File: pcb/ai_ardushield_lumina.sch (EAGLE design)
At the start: 90 parts, among them J1 1X02ST, J2 1X01, J3 1X06, J4 1X08, J5 1X08, J6 1X10, U1 ARDUINOUNOR3-STRAIGHT

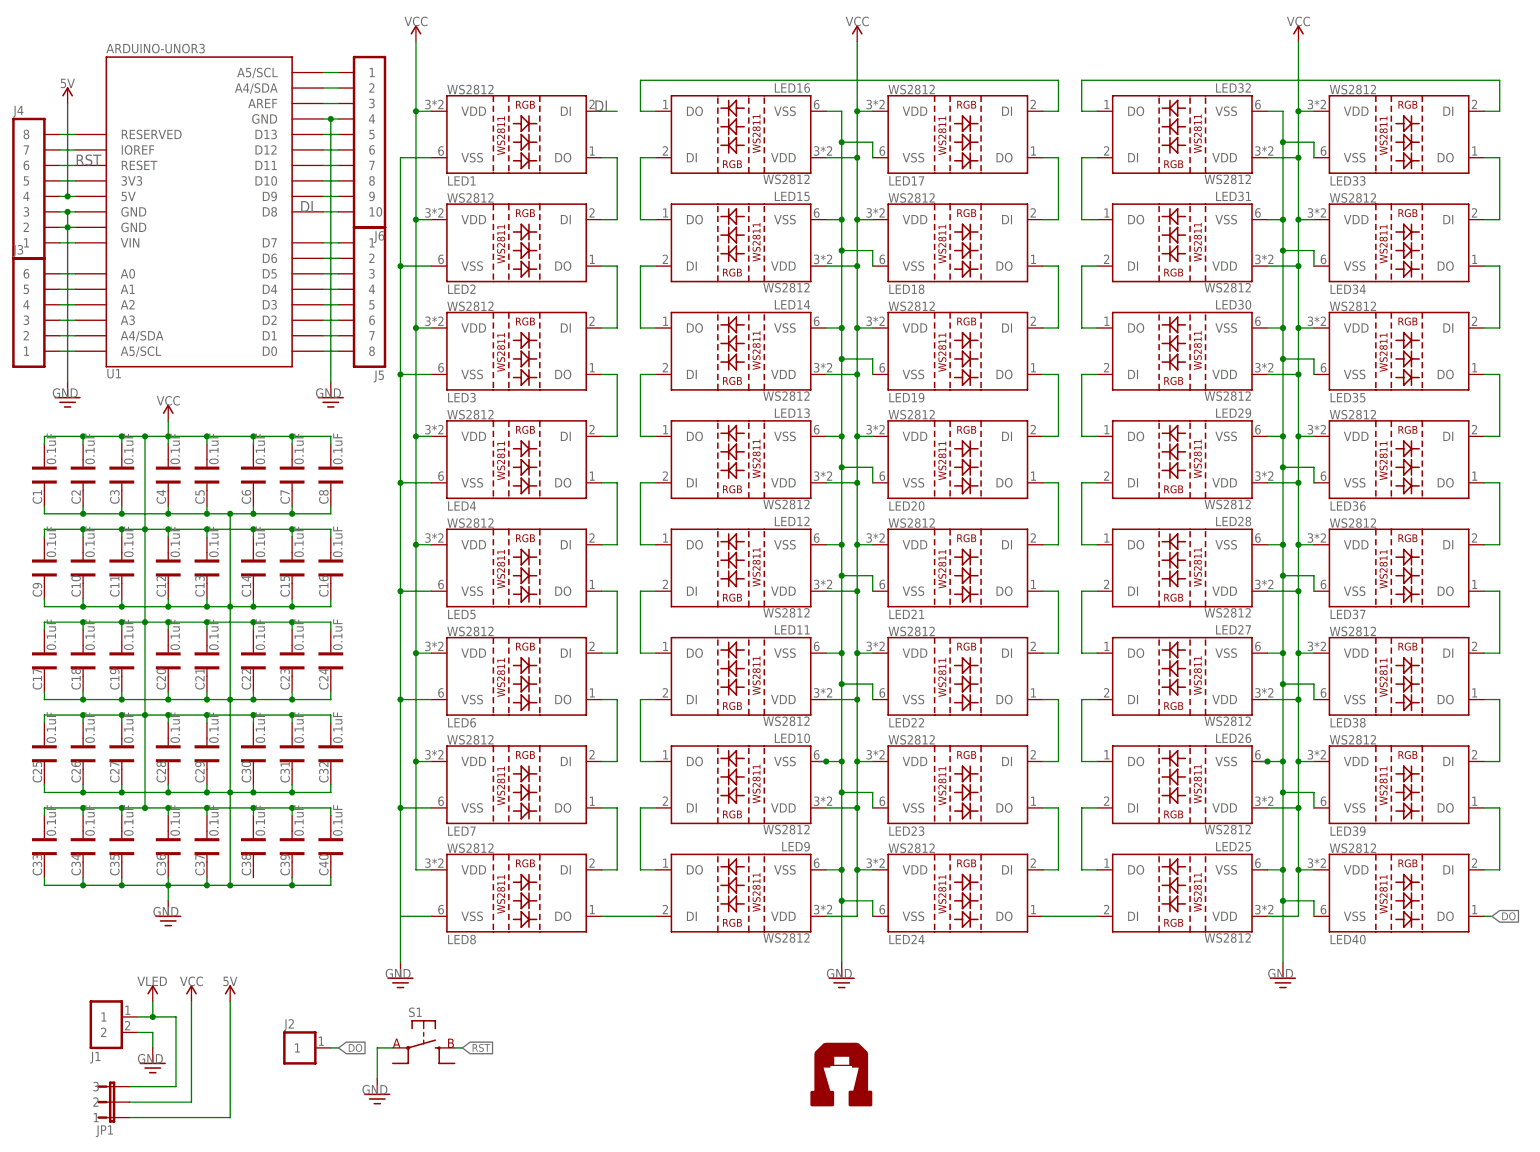
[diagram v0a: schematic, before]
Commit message: Modified the routing quite a bit.
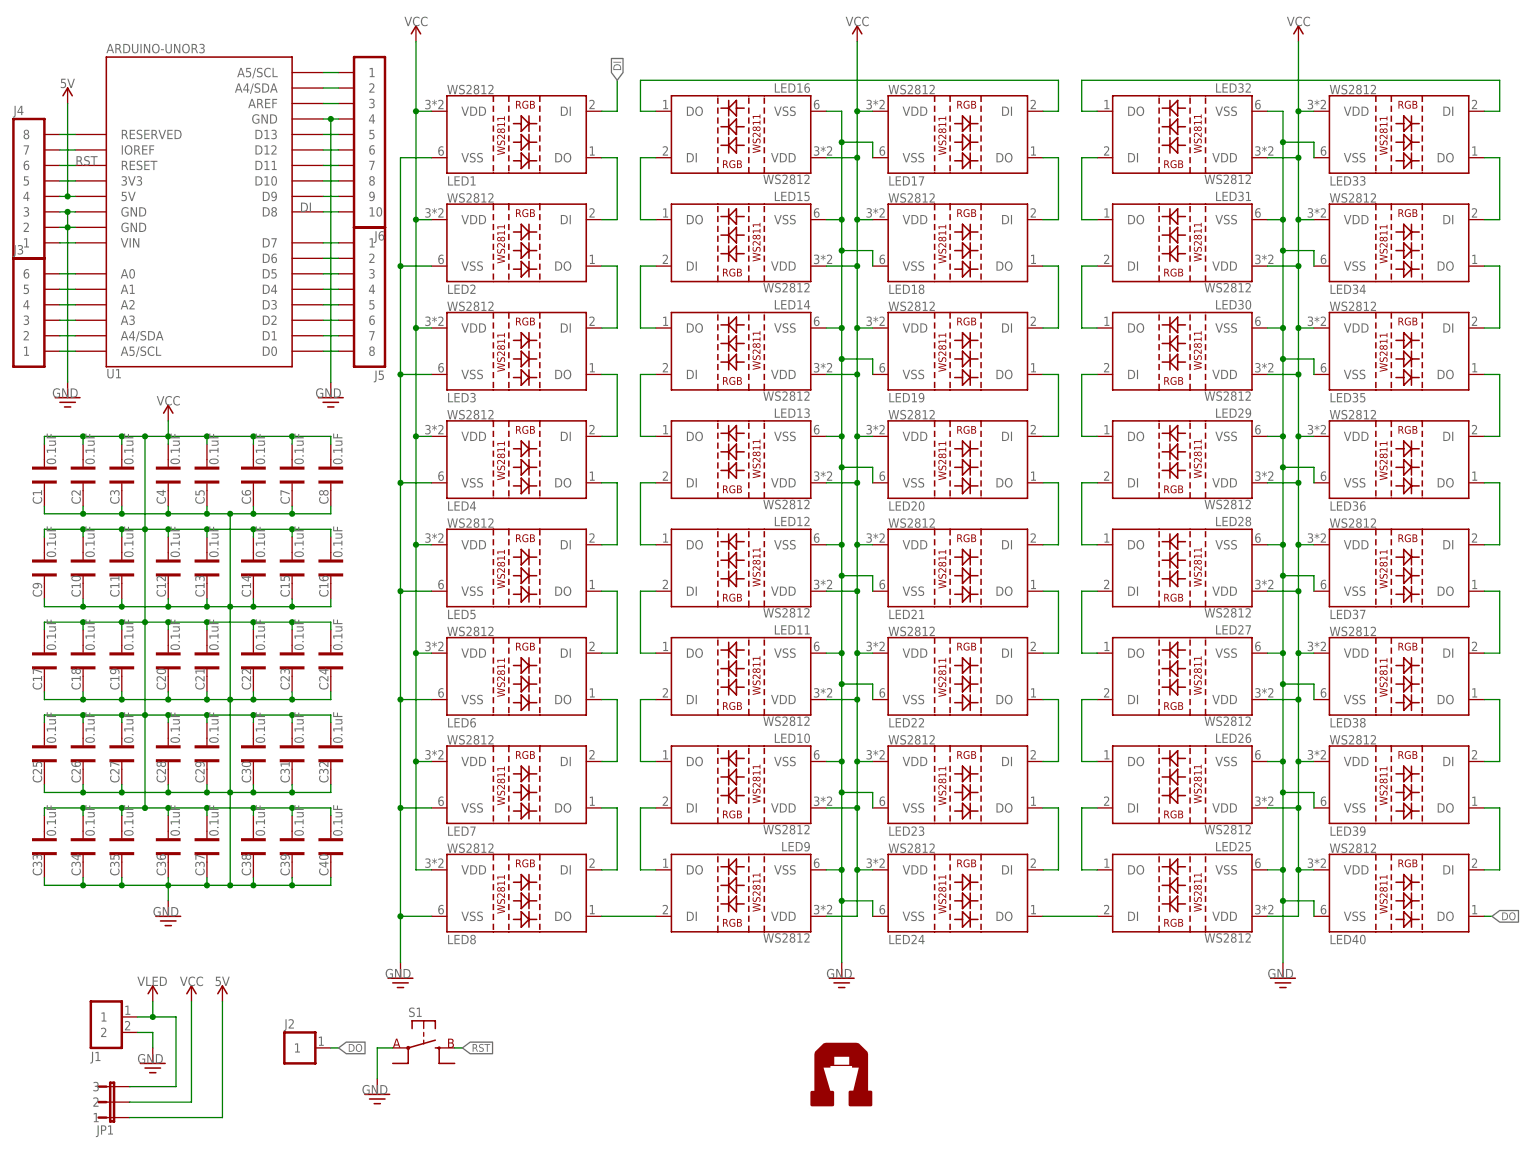
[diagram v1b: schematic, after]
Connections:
- removed net N$47: LED8.VSS
- net GND: now also C38.2, LED8.VSS
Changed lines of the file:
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@@
 <setting verticaltext="up"/>
 </settings>
-<grid distance="0.1" unitdist="inch" unit="inch" style="lines" multiple="1" display="no" altdistance="0.01" altunitdist="inch" altunit="inch"/>
+<grid distance="50" unitdist="mil" unit="mil" style="lines" multiple="1" display="yes" altdistance="0.01" altunitdist="inch" altunit="inch"/>
 <layers>
 <layer number="1" name="Top" color="4" fill="1" visible="no" active="no"/>
@@
 <layer number="111" name="LPC17xx" color="7" fill="1" visible="yes" active="yes"/>
 <layer number="112" name="tSilk" color="7" fill="1" visible="yes" active="yes"/>
+<layer number="113" name="Route13" color="7" fill="1" visible="no" active="no"/>
 <layer number="116" name="Patch_BOT" color="9" fill="4" visible="no" active="yes"/>
+<layer number="117" name="mPads" color="7" fill="1" visible="no" active="no"/>
+<layer number="118" name="mVias" color="7" fill="1" visible="no" active="no"/>
+<layer number="119" name="mUnrouted" color="7" fill="1" visible="no" active="no"/>
+<layer number="120" name="mDimension" color="7" fill="1" visible="no" active="no"/>
 <layer number="121" name="_tsilk" color="7" fill="1" visible="no" active="yes"/>
 <layer number="122" name="_bsilk" color="7" fill="1" visible="no" active="yes"/>
@@
 <layer number="127" name="_tValues" color="7" fill="1" visible="yes" active="yes"/>
 <layer number="128" name="_bValues" color="7" fill="1" visible="yes" active="yes"/>
+<layer number="129" name="mtStop" color="7" fill="1" visible="no" active="no"/>
+<layer number="130" name="mbStop" color="7" fill="1" visible="no" active="no"/>
 <layer number="131" name="tAdjust" color="7" fill="1" visible="no" active="yes"/>
 <layer number="132" name="bAdjust" color="7" fill="1" visible="no" active="yes"/>
+<layer number="133" name="mtFinish" color="7" fill="1" visible="no" active="no"/>
+<layer number="134" name="mbFinish" color="7" fill="1" visible="no" active="no"/>
+<layer number="135" name="mtGlue" color="7" fill="1" visible="no" active="no"/>
+<layer number="136" name="mbGlue" color="7" fill="1" visible="no" active="no"/>
+<layer number="137" name="mtTest" color="7" fill="1" visible="no" active="no"/>
+<layer number="138" name="mbTest" color="7" fill="1" visible="no" active="no"/>
+<layer number="139" name="mtKeepout" color="7" fill="1" visible="no" active="no"/>
+<layer number="140" name="mbKeepout" color="7" fill="1" visible="no" active="no"/>
+<layer number="141" name="mtRestrict" color="7" fill="1" visible="no" active="no"/>
+<layer number="142" name="mbRestrict" color="7" fill="1" visible="no" active="no"/>
+<layer number="143" name="mvRestrict" color="7" fill="1" visible="no" active="no"/>
 <layer number="144" name="Drill_legend" color="7" fill="1" visible="no" active="yes"/>
+<layer number="145" name="mHoles" color="7" fill="1" visible="no" active="no"/>
+<layer number="146" name="mMilling" color="7" fill="1" visible="no" active="no"/>
+<layer number="147" name="mMeasures" color="7" fill="1" visible="no" active="no"/>
+<layer number="148" name="mDocument" color="7" fill="1" visible="no" active="no"/>
+<layer number="149" name="mReference" color="7" fill="1" visible="no" active="no"/>
 <layer number="150" name="Notes" color="7" fill="1" visible="no" active="yes"/>
 <layer number="151" name="HeatSink" color="7" fill="1" visible="no" active="yes"/>
@@
 <layer number="154" name="FabDoc2" color="2" fill="1" visible="no" active="no"/>
 <layer number="155" name="FabDoc3" color="7" fill="15" visible="no" active="no"/>
+<layer number="191" name="mNets" color="7" fill="1" visible="no" active="no"/>
+<layer number="192" name="mBusses" color="7" fill="1" visible="no" active="no"/>
+<layer number="193" name="mPins" color="7" fill="1" visible="no" active="no"/>
+<layer number="194" name="mSymbols" color="7" fill="1" visible="no" active="no"/>
+<layer number="195" name="mNames" color="7" fill="1" visible="no" active="no"/>
+<layer number="196" name="mValues" color="7" fill="1" visible="no" active="no"/>
 <layer number="199" name="Contour" color="7" fill="1" visible="no" active="yes"/>
 <layer number="200" name="200bmp" color="1" fill="10" visible="no" active="yes"/>
@@
 <part name="FRAME1" library="Ai_Miscellany" deviceset="FRAME-LETTER" device="">
 <attribute name="AUTHOR" value="A.I. HARDWARE SITH LORDS"/>
-<attribute name="REV" value="1.0"/>
+<attribute name="REV" value="1.1"/>
 </part>
 <part name="U1" library="Ai_Boards" deviceset="ARDUINO" device="UNOR3-STRAIGHT" value="ARDUINOUNOR3-STRAIGHT"/>
@@
 <instance part="GND5" gate="GND" x="24.13" y="12.7"/>
 <instance part="U$6" gate="G$1" x="10.16" y="170.18"/>
-<instance part="U$7" gate="G$1" x="36.83" y="22.86"/>
+<instance part="U$7" gate="G$1" x="35.56" y="22.86"/>
 <instance part="U$8" gate="1" x="30.48" y="22.86" smashed="yes"/>
 <instance part="J3" gate="M06X1" x="3.81" y="137.16"/>
@@
 <wire x1="134.62" y1="151.13" x2="137.16" y2="151.13" width="0.1524" layer="91"/>
 <junction x="137.16" y="151.13"/>
-<wire x1="133.35" y1="62.23" x2="134.62" y2="62.23" width="0.1524" layer="91"/>
-<junction x="137.16" y="62.23"/>
 <pinref part="LED9" gate="U1" pin="VSS"/>
-<wire x1="134.62" y1="62.23" x2="137.16" y2="62.23" width="0.1524" layer="91"/>
 <wire x1="134.62" y1="44.45" x2="137.16" y2="44.45" width="0.1524" layer="91"/>
 <junction x="137.16" y="44.45"/>
@@
 <junction x="137.16" y="128.27"/>
 <pinref part="LED10" gate="U1" pin="VSS"/>
-<junction x="134.62" y="62.23"/>
+<wire x1="134.62" y1="62.23" x2="137.16" y2="62.23" width="0.1524" layer="91"/>
+<junction x="137.16" y="62.23"/>
 </segment>
 <segment>
@@
 <wire x1="64.77" y1="90.17" x2="64.77" y2="72.39" width="0.1524" layer="91"/>
 <wire x1="64.77" y1="72.39" x2="64.77" y2="54.61" width="0.1524" layer="91"/>
-<wire x1="64.77" y1="54.61" x2="64.77" y2="29.21" width="0.1524" layer="91"/>
+<wire x1="64.77" y1="54.61" x2="64.77" y2="36.83" width="0.1524" layer="91"/>
+<wire x1="64.77" y1="36.83" x2="64.77" y2="29.21" width="0.1524" layer="91"/>
 <wire x1="69.85" y1="54.61" x2="64.77" y2="54.61" width="0.1524" layer="91"/>
 <junction x="64.77" y="54.61"/>
@@
 <wire x1="69.85" y1="143.51" x2="64.77" y2="143.51" width="0.1524" layer="91"/>
 <junction x="64.77" y="143.51"/>
+<pinref part="LED8" gate="U1" pin="VSS"/>
+<wire x1="69.85" y1="36.83" x2="64.77" y2="36.83" width="0.1524" layer="91"/>
+<junction x="64.77" y="36.83"/>
 </segment>
 <segment>
@@
 <wire x1="207.01" y1="151.13" x2="209.55" y2="151.13" width="0.1524" layer="91"/>
 <junction x="209.55" y="151.13"/>
-<wire x1="205.74" y1="62.23" x2="207.01" y2="62.23" width="0.1524" layer="91"/>
-<junction x="209.55" y="62.23"/>
-<wire x1="207.01" y1="62.23" x2="209.55" y2="62.23" width="0.1524" layer="91"/>
 <wire x1="207.01" y1="44.45" x2="209.55" y2="44.45" width="0.1524" layer="91"/>
 <junction x="209.55" y="44.45"/>
 <pinref part="LED25" gate="U1" pin="VSS"/>
-<pinref part="LED26" gate="U1" pin="VSS"/>
-<junction x="207.01" y="62.23"/>
 <pinref part="LED27" gate="U1" pin="VSS"/>
 <pinref part="LED28" gate="U1" pin="VSS"/>
@@
 <wire x1="214.63" y1="146.05" x2="209.55" y2="146.05" width="0.1524" layer="91"/>
 <junction x="209.55" y="146.05"/>
+<pinref part="LED26" gate="U1" pin="VSS"/>
+<wire x1="207.01" y1="62.23" x2="209.55" y2="62.23" width="0.1524" layer="91"/>
+<junction x="209.55" y="62.23"/>
 </segment>
 <segment>
@@
 <wire x1="26.67" y1="41.91" x2="33.02" y2="41.91" width="0.1524" layer="91"/>
 <wire x1="33.02" y1="41.91" x2="36.83" y2="41.91" width="0.1524" layer="91"/>
-<wire x1="36.83" y1="41.91" x2="46.99" y2="41.91" width="0.1524" layer="91"/>
+<wire x1="36.83" y1="41.91" x2="40.64" y2="41.91" width="0.1524" layer="91"/>
+<wire x1="40.64" y1="41.91" x2="46.99" y2="41.91" width="0.1524" layer="91"/>
 <wire x1="46.99" y1="41.91" x2="53.34" y2="41.91" width="0.1524" layer="91"/>
 <wire x1="53.34" y1="41.91" x2="53.34" y2="43.18" width="0.1524" layer="91"/>
@@
 <junction x="12.7" y="102.87"/>
 <junction x="36.83" y="102.87"/>
+<pinref part="C38" gate="G$1" pin="2"/>
+<wire x1="40.64" y1="43.18" x2="40.64" y2="41.91" width="0.1524" layer="91"/>
+<junction x="40.64" y="41.91"/>
 </segment>
 <segment>
@@
 </segment>
 </net>
-<net name="N$47" class="0">
-<segment>
-<pinref part="LED8" gate="U1" pin="VSS"/>
-<wire x1="69.85" y1="36.83" x2="64.77" y2="36.83" width="0.1524" layer="91"/>
-</segment>
-</net>
 <net name="VLED" class="0">
 <segment>
@@
 <segment>
 <pinref part="JP1" gate="G$1" pin="1"/>
-<wire x1="20.32" y1="3.81" x2="36.83" y2="3.81" width="0.1524" layer="91"/>
-<wire x1="36.83" y1="3.81" x2="36.83" y2="22.86" width="0.1524" layer="91"/>
+<wire x1="20.32" y1="3.81" x2="35.56" y2="3.81" width="0.1524" layer="91"/>
+<wire x1="35.56" y1="3.81" x2="35.56" y2="22.86" width="0.1524" layer="91"/>
 <pinref part="U$7" gate="G$1" pin="5V"/>
 </segment>
@@
 <pinref part="J6" gate="M10X1" pin="10"/>
 <wire x1="54.61" y1="152.4" x2="52.07" y2="152.4" width="0.1524" layer="91"/>
-<label x="48.26" y="152.4" size="1.778" layer="95" ratio="15"/>
+<label x="48.26" y="152.4" size="1.524" layer="95" ratio="15"/>
 </segment>
 <segment>
 <pinref part="LED1" gate="U1" pin="DI"/>
 <wire x1="97.79" y1="168.91" x2="100.33" y2="168.91" width="0.1524" layer="91"/>
-<label x="96.52" y="168.91" size="1.778" layer="95" ratio="15"/>
+<label x="100.33" y="173.99" size="1.27" layer="95" ratio="15" rot="R90" xref="yes"/>
+<wire x1="100.33" y1="173.99" x2="100.33" y2="168.91" width="0.1524" layer="91"/>
 </segment>
 </net>
@@
 <pinref part="U1" gate="G$1" pin="RESET"/>
 <wire x1="8.89" y1="160.02" x2="11.43" y2="160.02" width="0.1524" layer="91"/>
-<label x="11.43" y="160.02" size="1.778" layer="95" ratio="15"/>
-</segment>
-</net>
+<label x="11.43" y="160.02" size="1.524" layer="95" ratio="15"/>
+</segment>
+</net>
